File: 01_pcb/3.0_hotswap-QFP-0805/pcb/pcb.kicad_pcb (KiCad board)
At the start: 2 copper layers, 256 x 75 mm, 126 parts, among them J1 TYPE-C-31-M12_13, J2 AVR-ISP-6_mod, J3 4PIN, J5 Conn_01x08, SW1 SW_PUSH, U1 ATmega32U4-A, U4 USBLC6-2SC6, Y1 16MHz

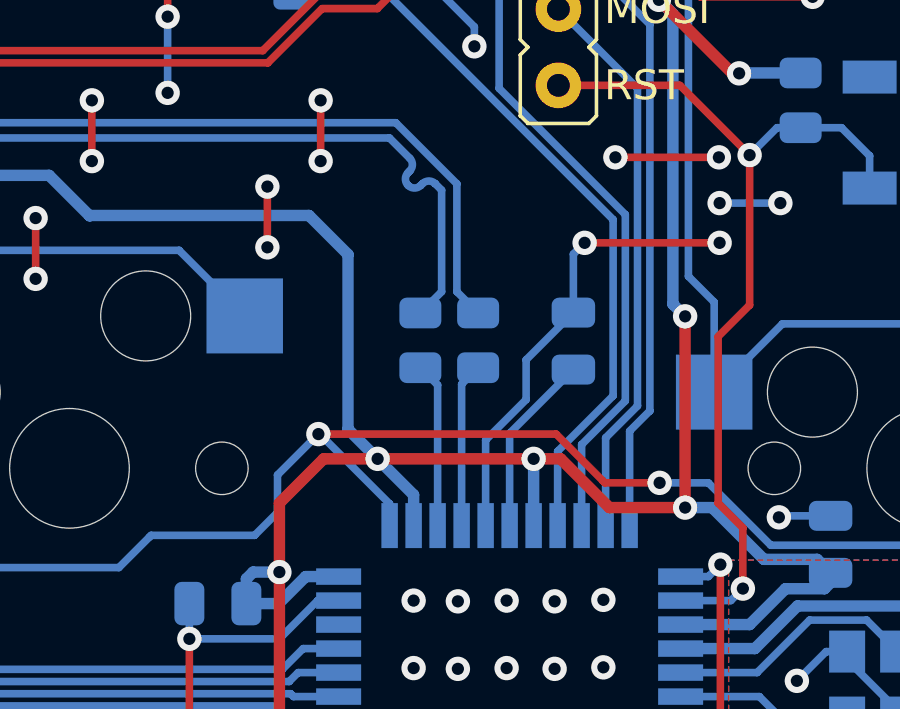
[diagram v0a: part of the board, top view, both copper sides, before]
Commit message: rename folders
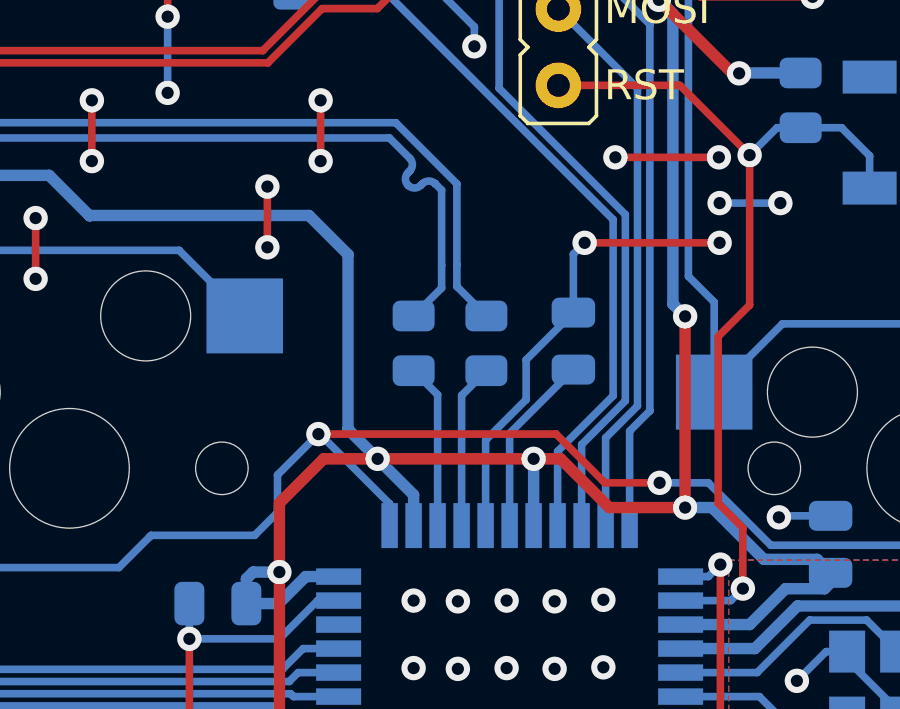
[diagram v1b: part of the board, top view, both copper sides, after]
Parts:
- moved R3 0.29 mm to (258.0, 44.6)
- moved R2 0.25 mm to (255.6, 44.6)
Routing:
- net D+: track 4.97 -> 5.50 mm
- net D-: track 4.98 -> 5.49 mm
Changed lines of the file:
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@@
   )
   (footprint "Resistor_SMD:R_0805_2012Metric" (layer "B.Cu")
-    (at 257.7 44.55 -90)
+    (at 257.975 44.65 -90)
     (descr "Resistor SMD 0805 (2012 Metric), square (rectangular) end terminal, IPC_7351 nominal, (Body size source: IPC-SM-782 page 72, https://www.pcb-3d.com/wordpress/wp-content/uploads/ipc-sm-782a_amendment_1_and_2.pdf), generated with kicad-footprint-generator")
     (tags "resistor")
@@
   )
   (footprint "Resistor_SMD:R_0805_2012Metric" (layer "B.Cu")
-    (at 255.775 44.55 90)
+    (at 255.55 44.65 90)
     (descr "Resistor SMD 0805 (2012 Metric), square (rectangular) end terminal, IPC_7351 nominal, (Body size source: IPC-SM-782 page 72, https://www.pcb-3d.com/wordpress/wp-content/uploads/ipc-sm-782a_amendment_1_and_2.pdf), generated with kicad-footprint-generator")
     (tags "resistor")
@@
   (segment (start 44.694788 40.404) (end 43.920999 39.630211) (width 0.254) (layer "B.Cu") (net 60))
   (segment (start 42.707849 28.487981) (end 42.707849 26.789085) (width 0.254) (layer "B.Cu") (net 60))
-  (segment (start 256.483499 39.542711) (end 256.483499 42.929001) (width 0.254) (layer "B.Cu") (net 60))
+  (segment (start 256.483499 39.542711) (end 256.483499 42.05) (width 0.254) (layer "B.Cu") (net 60))
   (segment (start 241.175 37.804001) (end 254.744789 37.804001) (width 0.254) (layer "B.Cu") (net 60))
   (segment (start 43.282263 37.65) (end 43.920999 37.011264) (width 0.254) (layer "B.Cu") (net 60))
@@
   (segment (start 43.920999 38.570999) (end 43 37.65) (width 0.254) (layer "B.Cu") (net 60))
   (segment (start 54.030211 37.804001) (end 51.430212 40.404) (width 0.254) (layer "B.Cu") (net 60))
-  (segment (start 256.483499 42.929001) (end 255.775 43.6375) (width 0.254) (layer "B.Cu") (net 60))
   (segment (start 42.707849 26.789085) (end 42.707849 26.577636) (width 0.2032) (layer "B.Cu") (net 60))
   (segment (start 238.475 37.804001) (end 54.030211 37.804001) (width 0.254) (layer "B.Cu") (net 60))
@@
   (segment (start 254.744789 37.804001) (end 255.420394 38.479606) (width 0.254) (layer "B.Cu") (net 60))
   (segment (start 255.789218 39.383573) (end 255.789217 39.383574) (width 0.254) (layer "B.Cu") (net 60))
+  (segment (start 256.483499 42.804001) (end 255.55 43.7375) (width 0.254) (layer "B.Cu") (net 60))
+  (segment (start 256.483499 42.05) (end 256.483499 42.804001) (width 0.254) (layer "B.Cu") (net 60))
   (segment (start 238.720999 38.05) (end 238.475 37.804001) (width 0.254) (layer "B.Cu") (net 60))
   (segment (start 239.9 38.05) (end 238.720999 38.05) (width 0.254) (layer "B.Cu") (net 60))
@@
   (arc (start 255.420394 38.479606) (mid 255.508262 38.691739) (end 255.420393 38.903871) (width 0.254) (layer "B.Cu") (net 60))
   (segment (start 44.905212 39.896) (end 51.219788 39.896) (width 0.254) (layer "B.Cu") (net 61))
-  (segment (start 256.991501 42.929001) (end 256.991501 39.332289) (width 0.254) (layer "B.Cu") (net 61))
+  (segment (start 256.991501 42.025) (end 256.991501 39.332289) (width 0.254) (layer "B.Cu") (net 61))
   (segment (start 45.067737 37.65) (end 44.429001 37.011264) (width 0.254) (layer "B.Cu") (net 61))
   (segment (start 239.9 37.05) (end 240.929001 37.05) (width 0.254) (layer "B.Cu") (net 61))
@@
   (segment (start 44.729001 30.975) (end 44.948693 30.975) (width 0.254) (layer "B.Cu") (net 61))
   (segment (start 44.948693 30.375) (end 44.729001 30.375) (width 0.254) (layer "B.Cu") (net 61))
+  (segment (start 256.991501 42.025) (end 256.991501 42.754001) (width 0.254) (layer "B.Cu") (net 61))
   (segment (start 44.429001 38.570999) (end 44.429001 39.419789) (width 0.254) (layer "B.Cu") (net 61))
   (segment (start 44.429001 30.009215) (end 44.429001 29.475) (width 0.254) (layer "B.Cu") (net 61))
@@
   (segment (start 51.219788 39.896) (end 53.819789 37.295999) (width 0.254) (layer "B.Cu") (net 61))
   (segment (start 44.729001 32.175) (end 44.948693 32.175) (width 0.254) (layer "B.Cu") (net 61))
-  (segment (start 257.7 43.6375) (end 256.991501 42.929001) (width 0.254) (layer "B.Cu") (net 61))
   (segment (start 70.05 37.295999) (end 238.525 37.295999) (width 0.254) (layer "B.Cu") (net 61))
   (segment (start 44.429001 39.419789) (end 44.905212 39.896) (width 0.254) (layer "B.Cu") (net 61))
   (segment (start 43.203849 28.249848) (end 43.7645 28.8105) (width 0.254) (layer "B.Cu") (net 61))
   (segment (start 44.429001 29.475) (end 43.7645 28.8105) (width 0.254) (layer "B.Cu") (net 61))
+  (segment (start 256.991501 42.754001) (end 257.975 43.7375) (width 0.254) (layer "B.Cu") (net 61))
   (arc (start 69.15 36.917639) (mid 69.237868 36.705507) (end 69.45 36.617639) (width 0.254) (layer "B.Cu") (net 61))
   (arc (start 69.75 36.995999) (mid 69.837868 37.208131) (end 70.05 37.295999) (width 0.254) (layer "B.Cu") (net 61))
@@
   (segment (start 254.125 64.25) (end 254.75 63.625) (width 0.254) (layer "B.Cu") (net 70))
   (segment (start 254.125 64.95) (end 254.125 64.25) (width 0.254) (layer "B.Cu") (net 70))
-  (segment (start 257.15 50.2) (end 257.15 46.0125) (width 0.254) (layer "B.Cu") (net 71))
-  (segment (start 257.15 46.0125) (end 257.7 45.4625) (width 0.254) (layer "B.Cu") (net 71))
-  (segment (start 256.35 46.0375) (end 255.775 45.4625) (width 0.254) (layer "B.Cu") (net 72))
-  (segment (start 256.35 50.2) (end 256.35 46.0375) (width 0.254) (layer "B.Cu") (net 72))
+  (segment (start 257.15 50.725) (end 257.15 46.3875) (width 0.254) (layer "B.Cu") (net 71))
+  (segment (start 257.15 46.3875) (end 257.975 45.5625) (width 0.254) (layer "B.Cu") (net 71))
+  (segment (start 256.35 46.3625) (end 255.55 45.5625) (width 0.254) (layer "B.Cu") (net 72))
+  (segment (start 256.35 50.725) (end 256.35 46.3625) (width 0.254) (layer "B.Cu") (net 72))
   (segment (start 42.225 28.975) (end 41.5 28.25) (width 0.254) (layer "F.Cu") (net 73))
   (segment (start 37.5 28.25) (end 41.5 28.25) (width 0.254) (layer "F.Cu") (net 73))
